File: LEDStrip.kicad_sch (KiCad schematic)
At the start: 5 parts, among them J801 WAGO 2065-100, J802 WAGO 2065-100, J803 WAGO 2065-100, U801 74AHC1G125

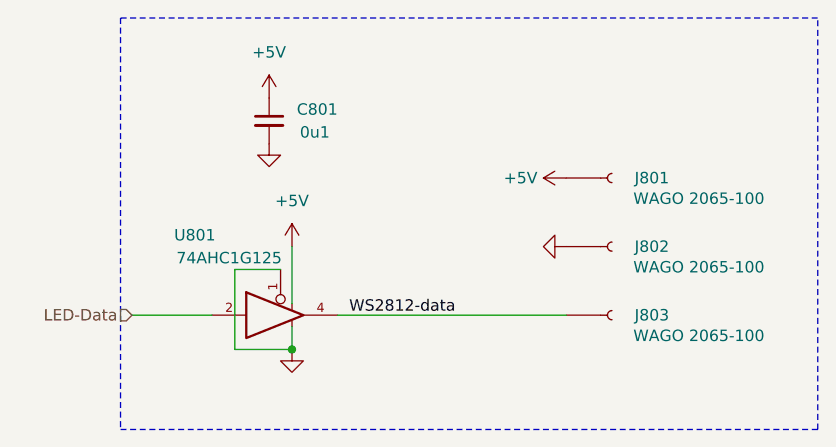
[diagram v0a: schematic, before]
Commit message: Refresh
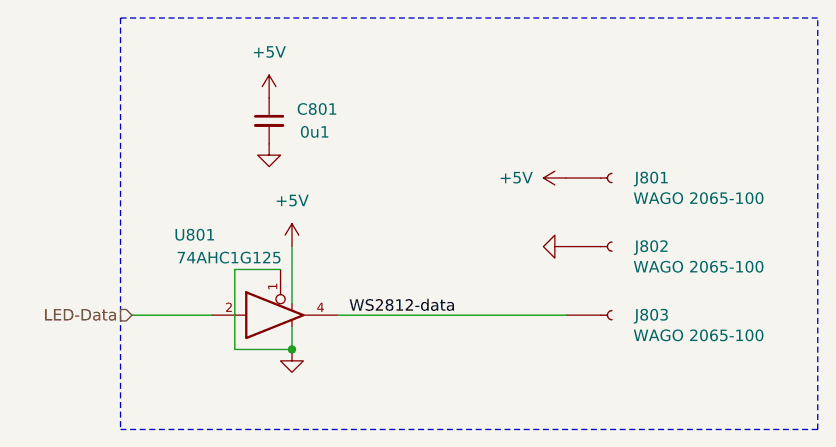
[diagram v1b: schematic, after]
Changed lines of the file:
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@@
 		(in_pos_files yes)
 		(dnp no)
-		(property "Reference" "#PWR0804"
+		(property "Reference" "#PWR804"
 			(at 161.29 107.95 0)
 			(hide yes)
@@
 			(project "drum"
 				(path "/6c8448b4-b04d-47e1-934e-e40cbe27a7be/48b625e4-a08e-4317-bdf1-f52549e397dd"
-					(reference "#PWR0804")
+					(reference "#PWR804")
 					(unit 1)
 				)
@@
 		(in_pos_files yes)
 		(dnp no)
-		(property "Reference" "#PWR0803"
+		(property "Reference" "#PWR803"
 			(at 171.45 100.33 0)
 			(hide yes)
@@
 		)
 		(property "Value" "+5V"
-			(at 162.56 100.33 90)
-			(show_name no)
-			(do_not_autoplace no)
-			(effects
-				(font
-					(size 1.27 1.27)
+			(at 162.052 100.33 90)
+			(show_name no)
+			(do_not_autoplace no)
+			(effects
+				(font
+					(size 1.27 1.27)
+					(color 255 92 187 1)
 				)
 			)
@@
 			(project "drum"
 				(path "/6c8448b4-b04d-47e1-934e-e40cbe27a7be/48b625e4-a08e-4317-bdf1-f52549e397dd"
-					(reference "#PWR0803")
+					(reference "#PWR803")
 					(unit 1)
 				)
@@
 		(in_pos_files yes)
 		(dnp no)
-		(property "Reference" "#PWR0806"
+		(property "Reference" "#PWR806"
 			(at 134.62 95.25 0)
 			(hide yes)
@@
 				(font
 					(size 1.27 1.27)
+					(color 255 92 187 1)
 				)
 			)
@@
 			(project "drum"
 				(path "/6c8448b4-b04d-47e1-934e-e40cbe27a7be/48b625e4-a08e-4317-bdf1-f52549e397dd"
-					(reference "#PWR0806")
+					(reference "#PWR806")
 					(unit 1)
 				)
@@
 		(in_pos_files yes)
 		(dnp no)
-		(property "Reference" "#PWR0801"
+		(property "Reference" "#PWR801"
 			(at 137.16 111.76 0)
 			(hide yes)
@@
 				(font
 					(size 1.27 1.27)
+					(color 255 92 187 1)
 				)
 			)
@@
 			(project "drum"
 				(path "/6c8448b4-b04d-47e1-934e-e40cbe27a7be/48b625e4-a08e-4317-bdf1-f52549e397dd"
-					(reference "#PWR0801")
+					(reference "#PWR801")
 					(unit 1)
 				)
@@
 		(in_pos_files yes)
 		(dnp no)
-		(property "Reference" "#PWR0802"
+		(property "Reference" "#PWR802"
 			(at 137.16 125.73 0)
 			(hide yes)
@@
 			(project "drum"
 				(path "/6c8448b4-b04d-47e1-934e-e40cbe27a7be/48b625e4-a08e-4317-bdf1-f52549e397dd"
-					(reference "#PWR0802")
+					(reference "#PWR802")
 					(unit 1)
 				)
@@
 		(in_pos_files yes)
 		(dnp no)
-		(property "Reference" "#PWR0805"
+		(property "Reference" "#PWR805"
 			(at 134.62 102.87 0)
 			(hide yes)
@@
 			(project "drum"
 				(path "/6c8448b4-b04d-47e1-934e-e40cbe27a7be/48b625e4-a08e-4317-bdf1-f52549e397dd"
-					(reference "#PWR0805")
+					(reference "#PWR805")
 					(unit 1)
 				)
